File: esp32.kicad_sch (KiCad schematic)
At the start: 21 parts, among them J5 Micro SD card, U7 ESP32-WROVER

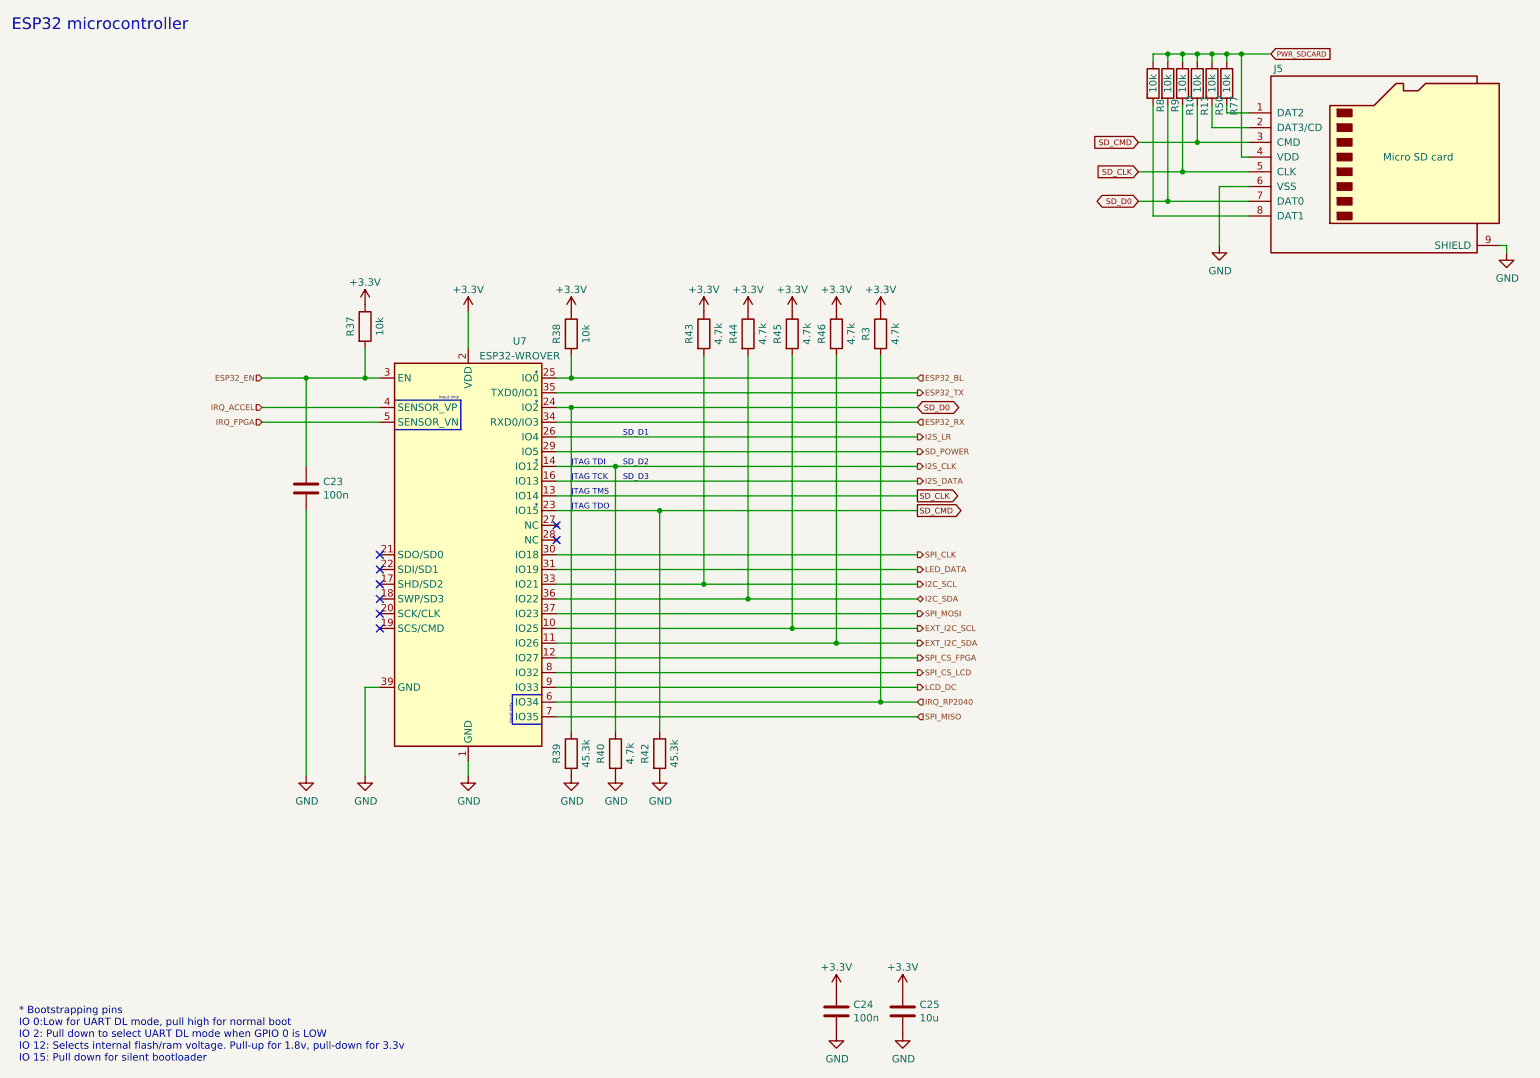
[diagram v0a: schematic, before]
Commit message: Remove user I2C bus, connect LCD control signals to ESP32 directly, replace I2S dac
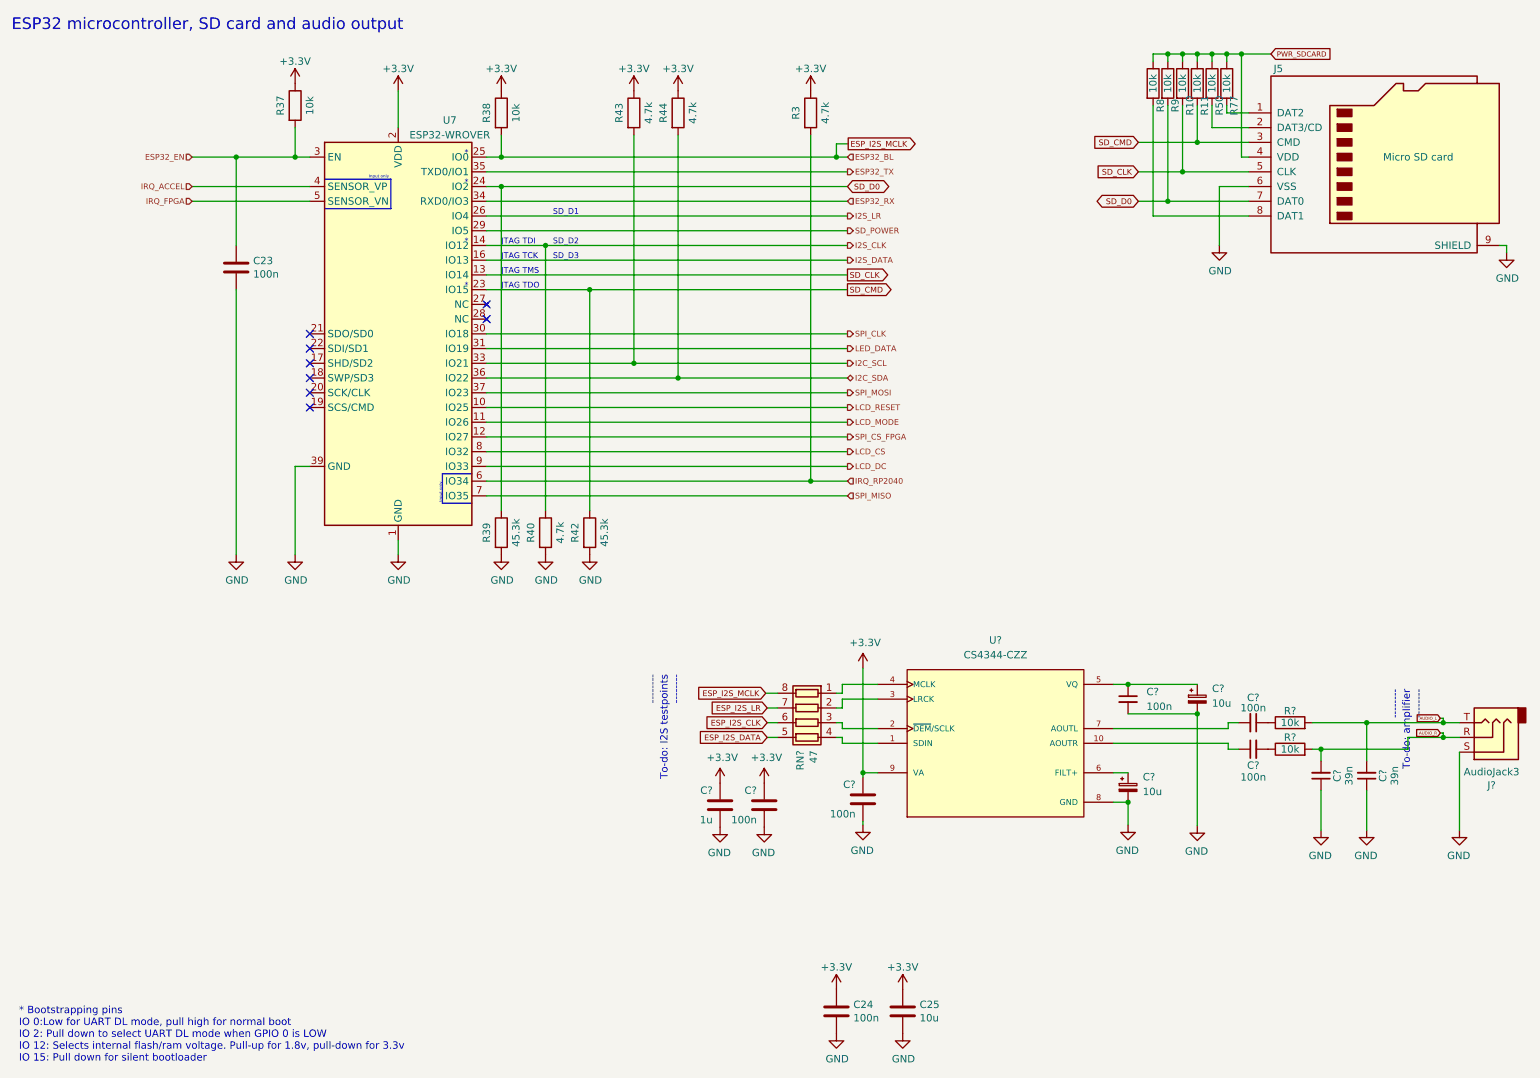
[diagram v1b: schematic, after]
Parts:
- removed R45, R46: 4.7k, Resistor_SMD:R_0402_1005Metric, symbol mch2021-rescue:R-Device
- added C? (x2): 100n, Capacitor_SMD:C_0402_1005Metric, symbol mch2021-rescue:C-Device
- added C? (x2): 39n, symbol Device:C_Small
- added C? (x3): 100n, symbol Device:C_Small
- added C?: 1u, Capacitor_SMD:C_0402_1005Metric, symbol mch2021-rescue:C-Device
- added C? (x2): 10u, symbol Device:C_Polarized_Small
- added J?: AudioJack3, custom:Boom-audiojack-PJ-320B, symbol mch2021-rescue:AudioJack3-Connector
- added R? (x2): 10k, Resistor_SMD:R_0402_1005Metric, symbol mch2021-rescue:R-Device
- added RN?: 47, Resistor_SMD:R_Array_Convex_4x0603, symbol mch2021-rescue:R_Pack04-Device
- added U?: CS4344-CZZ, SOP50P490X110-10N, symbol CS4344-CZZ:CS4344-CZZ
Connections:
- net +3V3: now also C?.1, C?.1, C?.1, U?.9 (VA)
- net GND: now also C?.1, C?.1, C?.2, C?.2, C?.2, C?.2, C?.2, C?.2, J?.S, U?.8 (GND)
- net ESP32_BL renamed ESP_I2S_MCLK
- net ESP_I2S_MCLK: now also RN?.8 (R1.2)
- net EXT_I2C_SCL renamed LCD_RESET
- net EXT_I2C_SDA renamed LCD_MODE
- net SPI_CS_LCD renamed LCD_CS
- new net: RN?.4 (R4.1), U?.1 (SDIN)
- new net: C?.1, U?.10 (AOUTR)
- new net: RN?.3 (R3.1), U?.2 (~{DEM}/SCLK)
- new net: RN?.2 (R2.1), U?.3 (LRCK)
- new net: RN?.1 (R1.1), U?.4 (MCLK)
- new net: C?.1, C?.1, U?.5 (VQ)
- new net: C?.1, U?.6 (FILT+)
- new net: C?.2, U?.7 (AOUTL)
- new net: C?.1, R?.1
- new net: C?.2, R?.1
- new net AUDIO_L: C?.2, J?.T, R?.2
- new net AUDIO_R: C?.2, J?.R, R?.2
- new net ESP_I2S_CLK: RN?.6 (R3.2)
- new net ESP_I2S_DATA: RN?.5 (R4.2)
- new net ESP_I2S_LR: RN?.7 (R2.2)
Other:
- note added: "-------- To-do: I2S testpoints --------"
- note added: "-------- To-do: amplifier --------"
- note added: "ESP32 microcontroller, SD card and audio output"
- note removed: "ESP32 microcontroller"
- moved on the sheet: C23, R3, R37, R38, R39, R40, R42, R43, R44, U7
